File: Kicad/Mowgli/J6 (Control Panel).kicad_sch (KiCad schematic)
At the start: 71 parts, among them J6 Control Panel, Q2 NMOS_G15, Q4 NMOS_G15, Q5 NMOS_G15, Q6 NMOS_G15, U2 STM32F030R8T6, U3 AMS1117-3.3

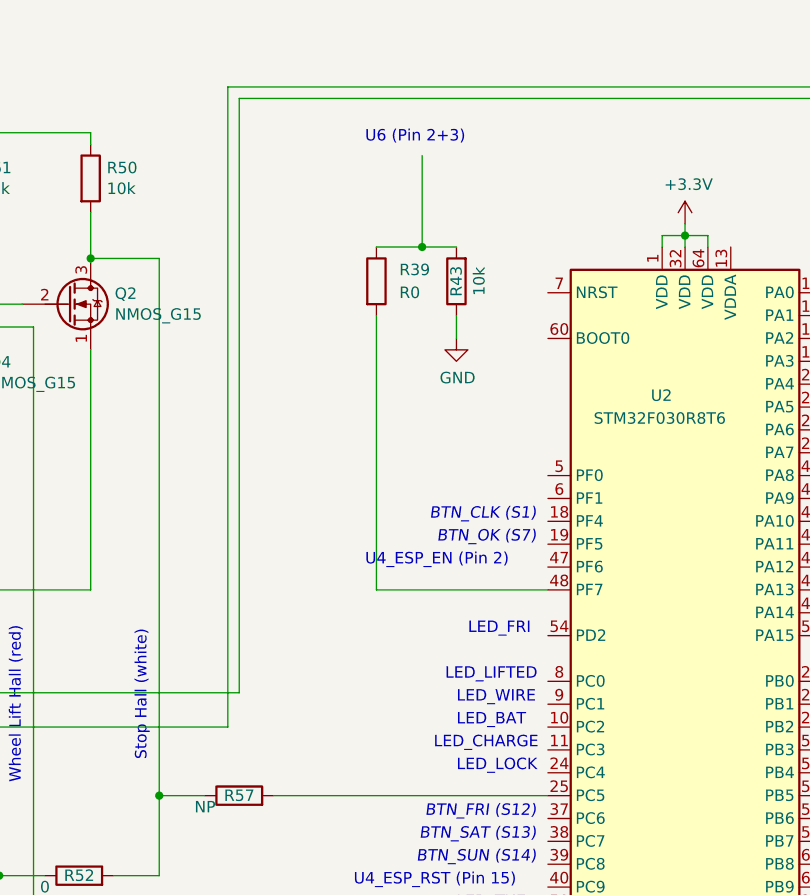
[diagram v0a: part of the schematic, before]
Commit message: Cleanup
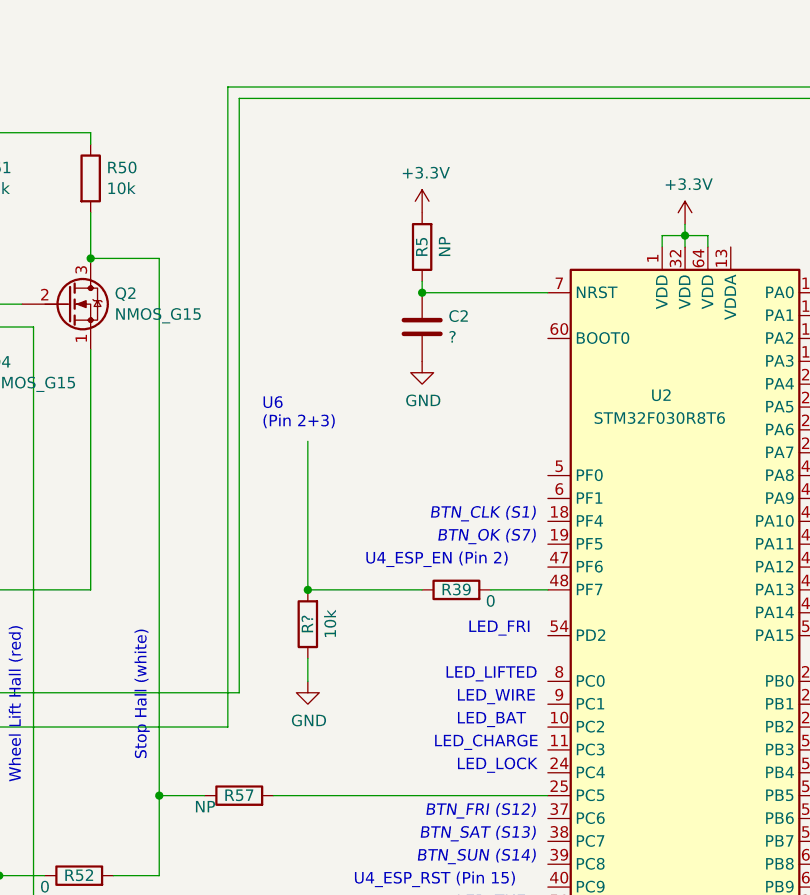
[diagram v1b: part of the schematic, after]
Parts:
- removed R43: 10k, symbol Device:R
- added C2: ?, symbol Device:C
- added R5: NP, symbol Device:R
- added R?: 10k, symbol Device:R
- R39: value R0 -> 0; now left out of the parts list
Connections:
- net +3.3V: now also R5.2
- net GND: now also C2.2, R?.1
- net at U2.7 (NRST): now also C2.1, R5.1
- net at R39.1: now also R?.2
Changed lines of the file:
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@@
   (junction (at 140.97 26.67) (diameter 0) (color 0 0 0 0)
   )
-  (junction (at 191.77 39.37) (diameter 0) (color 0 0 0 0)
-  )
   (junction (at 256.54 142.24) (diameter 0) (color 0 0 0 0)
   )
@@
   (junction (at 88.9 58.42) (diameter 0) (color 0 0 0 0)
   )
+  (junction (at 191.77 44.45) (diameter 0) (color 0 0 0 0)
+  )
   (junction (at 167.64 154.94) (diameter 0) (color 0 0 0 0)
   )
@@
   (junction (at 58.42 171.45) (diameter 0) (color 0 0 0 0)
   )
+  (junction (at 179.07 77.47) (diameter 0) (color 0 0 0 0)
+  )
   (junction (at 140.97 48.26) (diameter 0) (color 0 0 0 0)
   )
@@
     (stroke (width 0) (type default) (color 0 0 0 0))
   )
+  (wire (pts (xy 191.77 44.45) (xy 205.74 44.45))
+    (stroke (width 0) (type default) (color 0 0 0 0))
+  )
   (wire (pts (xy 101.6 119.38) (xy 101.6 111.76))
     (stroke (width 0) (type default) (color 0 0 0 0))
@@
     (stroke (width 0) (type default) (color 0 0 0 0))
   )
-  (wire (pts (xy 191.77 39.37) (xy 195.58 39.37))
-    (stroke (width 0) (type default) (color 0 0 0 0))
-  )
   (wire (pts (xy 274.32 147.32) (xy 274.32 152.4))
     (stroke (width 0) (type default) (color 0 0 0 0))
@@
     (stroke (width 0) (type default) (color 0 0 0 0))
   )
-  (wire (pts (xy 186.69 46.99) (xy 186.69 77.47))
-    (stroke (width 0) (type default) (color 0 0 0 0))
-  )
   (wire (pts (xy 220.98 132.08) (xy 220.98 133.35))
     (stroke (width 0) (type default) (color 0 0 0 0))
@@
     (stroke (width 0) (type default) (color 0 0 0 0))
   )
+  (wire (pts (xy 179.07 60.96) (xy 179.07 77.47))
+    (stroke (width 0) (type default) (color 0 0 0 0))
+  )
   (wire (pts (xy 125.73 162.56) (xy 125.73 173.99))
     (stroke (width 0) (type default) (color 0 0 0 0))
@@
     (stroke (width 0) (type default) (color 0 0 0 0))
   )
-  (wire (pts (xy 186.69 77.47) (xy 205.74 77.47))
+  (wire (pts (xy 179.07 77.47) (xy 191.77 77.47))
     (stroke (width 0) (type default) (color 0 0 0 0))
   )
@@
     (stroke (width 0) (type default) (color 0 0 0 0))
   )
-  (wire (pts (xy 186.69 39.37) (xy 191.77 39.37))
-    (stroke (width 0) (type default) (color 0 0 0 0))
-  )
   (wire (pts (xy 104.14 119.38) (xy 101.6 119.38))
     (stroke (width 0) (type default) (color 0 0 0 0))
@@
     (stroke (width 0) (type default) (color 0 0 0 0))
   )
+  (wire (pts (xy 199.39 77.47) (xy 205.74 77.47))
+    (stroke (width 0) (type default) (color 0 0 0 0))
+  )
+  (wire (pts (xy 179.07 85.09) (xy 179.07 87.63))
+    (stroke (width 0) (type default) (color 0 0 0 0))
+  )
   (wire (pts (xy 88.9 73.66) (xy 88.9 66.04))
     (stroke (width 0) (type default) (color 0 0 0 0))
@@
     (stroke (width 0) (type default) (color 0 0 0 0))
   )
+  (wire (pts (xy 191.77 43.18) (xy 191.77 44.45))
+    (stroke (width 0) (type default) (color 0 0 0 0))
+  )
   (wire (pts (xy 275.59 110.49) (xy 278.13 110.49))
     (stroke (width 0) (type default) (color 0 0 0 0))
@@
     (stroke (width 0) (type default) (color 0 0 0 0))
   )
-  (wire (pts (xy 195.58 46.99) (xy 195.58 49.53))
-    (stroke (width 0) (type default) (color 0 0 0 0))
-  )
   (wire (pts (xy 236.22 107.95) (xy 254 107.95))
     (stroke (width 0) (type default) (color 0 0 0 0))
@@
     (stroke (width 0) (type default) (color 0 0 0 0))
   )
-  (wire (pts (xy 191.77 29.21) (xy 191.77 39.37))
-    (stroke (width 0) (type default) (color 0 0 0 0))
-  )
   (wire (pts (xy 254 92.71) (xy 251.46 92.71))
     (stroke (width 0) (type default) (color 0 0 0 0))
@@
     (effects (font (size 1.27 1.27)) (justify left bottom))
   )
-  (text "U6 (Pin 2+3)" (at 185.42 27.94 0)
+  (text "U6\n(Pin 2+3)" (at 173.99 59.69 0)
     (effects (font (size 1.27 1.27)) (justify left bottom))
   )
@@
     (pin "2")
   )
+  (symbol (lib_id "Device:R") (at 179.07 81.28 180) (unit 1)
+    (in_bom yes) (on_board yes)
+    (property "Reference" "R?" (id 0) (at 179.07 81.28 90))
+    (property "Value" "10k" (id 1) (at 181.61 81.28 90))
+    (property "Footprint" "" (id 2) (at 180.848 81.28 90)
+      (effects (font (size 1.27 1.27)) hide)
+    )
+    (property "Datasheet" "~" (id 3) (at 179.07 81.28 0)
+      (effects (font (size 1.27 1.27)) hide)
+    )
+    (pin "1")
+    (pin "2")
+  )
   (symbol (lib_id "Device:D") (at 255.27 147.32 180) (unit 1)
     (in_bom yes) (on_board yes)
@@
     (pin "2")
   )
+  (symbol (lib_id "Device:R") (at 191.77 39.37 180) (unit 1)
+    (in_bom yes) (on_board yes)
+    (property "Reference" "R5" (id 0) (at 191.77 39.37 90))
+    (property "Value" "NP" (id 1) (at 194.31 39.37 90))
+    (property "Footprint" "" (id 2) (at 193.548 39.37 90)
+      (effects (font (size 1.27 1.27)) hide)
+    )
+    (property "Datasheet" "~" (id 3) (at 191.77 39.37 0)
+      (effects (font (size 1.27 1.27)) hide)
+    )
+    (pin "1")
+    (pin "2")
+  )
   (symbol (lib_id "power:GND") (at 274.32 157.48 0) (unit 1)
     (in_bom yes) (on_board yes)
@@
     (pin "1")
     (pin "2")
+  )
+  (symbol (lib_id "Device:C") (at 191.77 48.26 0) (unit 1)
+    (in_bom yes) (on_board yes)
+    (property "Reference" "C2" (id 0) (at 194.691 47.0916 0)
+      (effects (font (size 1.27 1.27)) (justify left))
+    )
+    (property "Value" "?" (id 1) (at 194.691 49.403 0)
+      (effects (font (size 1.27 1.27)) (justify left))
+    )
+    (property "Footprint" "" (id 2) (at 192.7352 52.07 0)
+      (effects (font (size 1.27 1.27)) hide)
+    )
+    (property "Datasheet" "~" (id 3) (at 191.77 48.26 0)
+      (effects (font (size 1.27 1.27)) hide)
+    )
+    (pin "1")
+    (pin "2")
+  )
+  (symbol (lib_id "power:+3.3V") (at 191.77 35.56 0) (unit 1)
+    (in_bom yes) (on_board yes)
+    (property "Reference" "#PWR?" (id 0) (at 191.77 39.37 0)
+      (effects (font (size 1.27 1.27)) hide)
+    )
+    (property "Value" "+3.3V" (id 1) (at 192.151 31.1658 0))
+    (property "Footprint" "" (id 2) (at 191.77 35.56 0)
+      (effects (font (size 1.27 1.27)) hide)
+    )
+    (property "Datasheet" "" (id 3) (at 191.77 35.56 0)
+      (effects (font (size 1.27 1.27)) hide)
+    )
+    (pin "1")
   )
   (symbol (lib_id "Device:R") (at 257.81 92.71 90) (unit 1)
@@
     )
     (property "Datasheet" "" (id 3) (at 281.94 45.72 0)
+      (effects (font (size 1.27 1.27)) hide)
+    )
+    (pin "1")
+  )
+  (symbol (lib_id "power:GND") (at 191.77 52.07 0) (unit 1)
+    (in_bom yes) (on_board yes)
+    (property "Reference" "#PWR?" (id 0) (at 191.77 58.42 0)
+      (effects (font (size 1.27 1.27)) hide)
+    )
+    (property "Value" "GND" (id 1) (at 191.897 56.4642 0))
+    (property "Footprint" "" (id 2) (at 191.77 52.07 0)
+      (effects (font (size 1.27 1.27)) hide)
+    )
+    (property "Datasheet" "" (id 3) (at 191.77 52.07 0)
       (effects (font (size 1.27 1.27)) hide)
     )
@@
     (pin "2")
   )
+  (symbol (lib_id "power:GND") (at 179.07 87.63 0) (unit 1)
+    (in_bom yes) (on_board yes)
+    (property "Reference" "#PWR?" (id 0) (at 179.07 93.98 0)
+      (effects (font (size 1.27 1.27)) hide)
+    )
+    (property "Value" "GND" (id 1) (at 179.197 92.0242 0))
+    (property "Footprint" "" (id 2) (at 179.07 87.63 0)
+      (effects (font (size 1.27 1.27)) hide)
+    )
+    (property "Datasheet" "" (id 3) (at 179.07 87.63 0)
+      (effects (font (size 1.27 1.27)) hide)
+    )
+    (pin "1")
+  )
   (symbol (lib_id "Device:R") (at 260.35 38.1 270) (unit 1)
     (in_bom yes) (on_board yes)
@@
     (pin "2")
   )
-  (symbol (lib_id "power:GND") (at 195.58 49.53 0) (unit 1)
-    (in_bom yes) (on_board yes)
-    (property "Reference" "#PWR?" (id 0) (at 195.58 55.88 0)
-      (effects (font (size 1.27 1.27)) hide)
-    )
-    (property "Value" "GND" (id 1) (at 195.707 53.9242 0))
-    (property "Footprint" "" (id 2) (at 195.58 49.53 0)
-      (effects (font (size 1.27 1.27)) hide)
-    )
-    (property "Datasheet" "" (id 3) (at 195.58 49.53 0)
-      (effects (font (size 1.27 1.27)) hide)
-    )
-    (pin "1")
-  )
-  (symbol (lib_id "Device:R") (at 195.58 43.18 180) (unit 1)
-    (in_bom yes) (on_board yes)
-    (property "Reference" "R43" (id 0) (at 195.58 43.18 90))
-    (property "Value" "10k" (id 1) (at 198.12 43.18 90))
-    (property "Footprint" "" (id 2) (at 197.358 43.18 90)
-      (effects (font (size 1.27 1.27)) hide)
-    )
-    (property "Datasheet" "~" (id 3) (at 195.58 43.18 0)
-      (effects (font (size 1.27 1.27)) hide)
-    )
-    (pin "1")
-    (pin "2")
-  )
   (symbol (lib_id "Device:LED") (at 267.97 27.94 180) (unit 1)
     (in_bom yes) (on_board yes)
@@
     )
     (property "Datasheet" "~" (id 3) (at 267.97 27.94 0)
-      (effects (font (size 1.27 1.27)) hide)
-    )
-    (pin "1")
-    (pin "2")
-  )
-  (symbol (lib_id "Device:R") (at 186.69 43.18 0) (unit 1)
-    (in_bom yes) (on_board yes) (fields_autoplaced)
-    (property "Reference" "R39" (id 0) (at 189.23 41.9099 0)
-      (effects (font (size 1.27 1.27)) (justify left))
-    )
-    (property "Value" "R0" (id 1) (at 189.23 44.4499 0)
-      (effects (font (size 1.27 1.27)) (justify left))
-    )
-    (property "Footprint" "" (id 2) (at 184.912 43.18 90)
-      (effects (font (size 1.27 1.27)) hide)
-    )
-    (property "Datasheet" "~" (id 3) (at 186.69 43.18 0)
       (effects (font (size 1.27 1.27)) hide)
     )
@@
       (effects (font (size 1.27 1.27)) hide)
     )
+    (pin "1")
+    (pin "2")
+  )
+  (symbol (lib_id "Device:R") (at 195.58 77.47 90) (unit 1)
+    (in_bom no) (on_board no)
+    (property "Reference" "R39" (id 0) (at 195.58 77.47 90))
+    (property "Value" "0" (id 1) (at 199.39 78.74 90))
+    (property "Footprint" "" (id 2) (at 195.58 79.248 90)
+      (effects (font (size 1.27 1.27)) hide)
+    )
+    (property "Datasheet" "~" (id 3) (at 195.58 77.47 0)
+      (effects (font (size 1.27 1.27)) hide)
+    )
